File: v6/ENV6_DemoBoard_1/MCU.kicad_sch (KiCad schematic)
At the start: 44 parts, among them J1 Pico Debugger (SWD), J201 Conn_01x04, U101 RP2354B, U102 W25Q16JVUXIQ, U103 Pi-Radio, Y101 KX7_QRZ

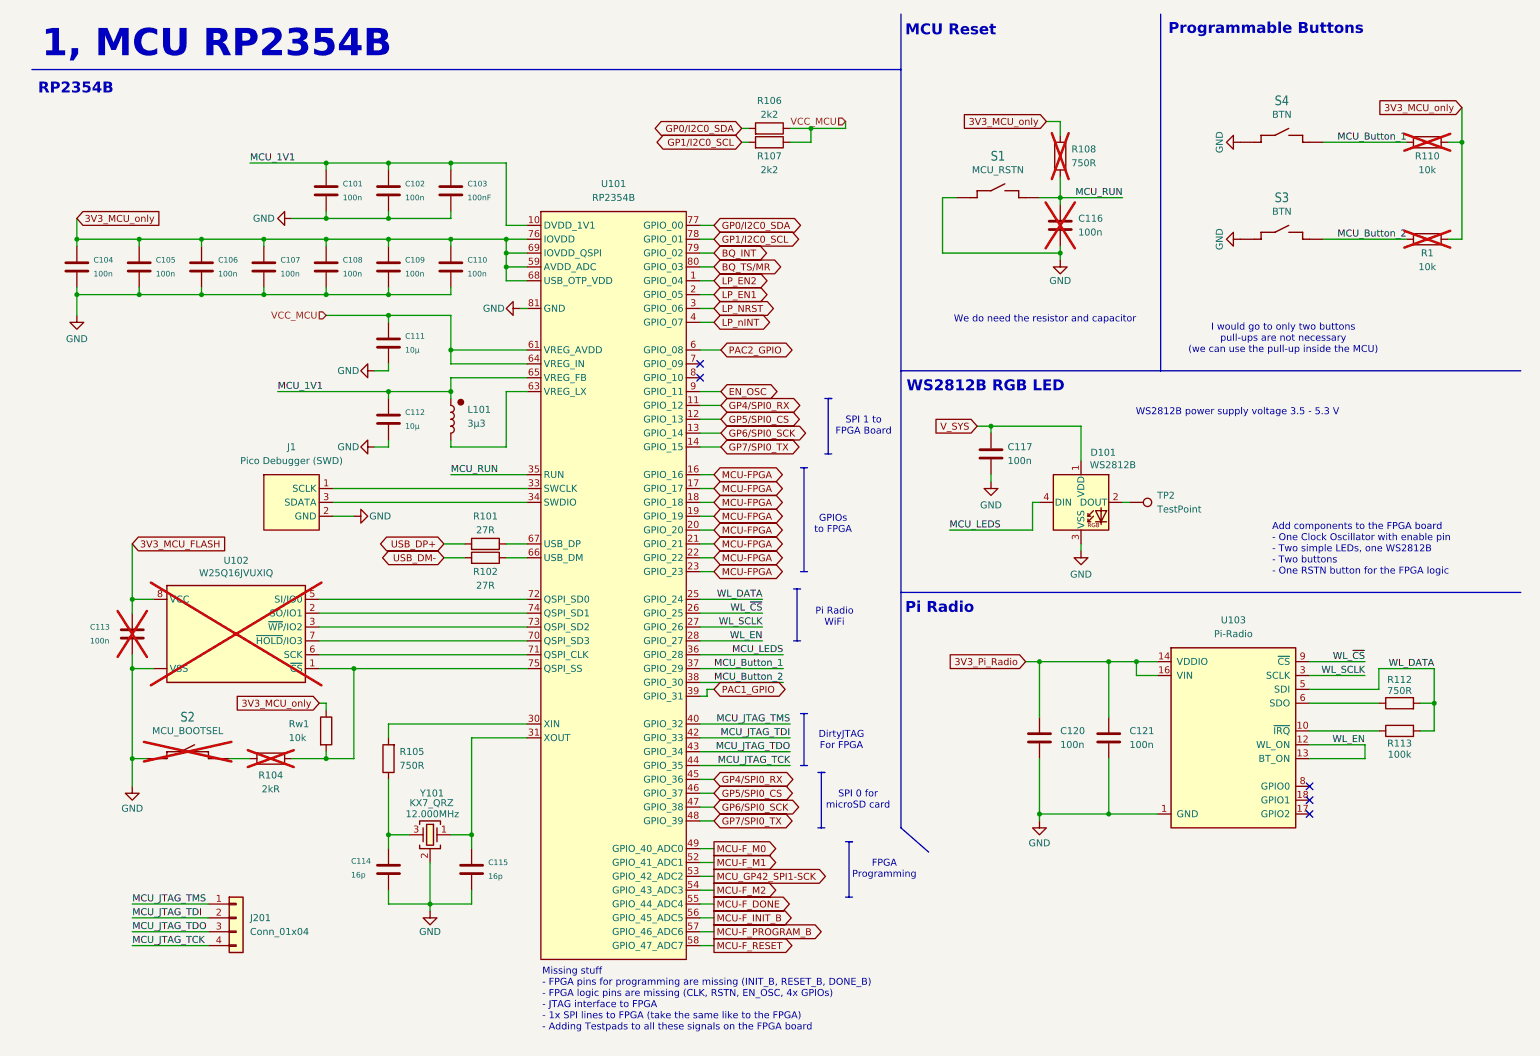
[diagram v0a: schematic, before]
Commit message: Changes after second rev of ENV6 test
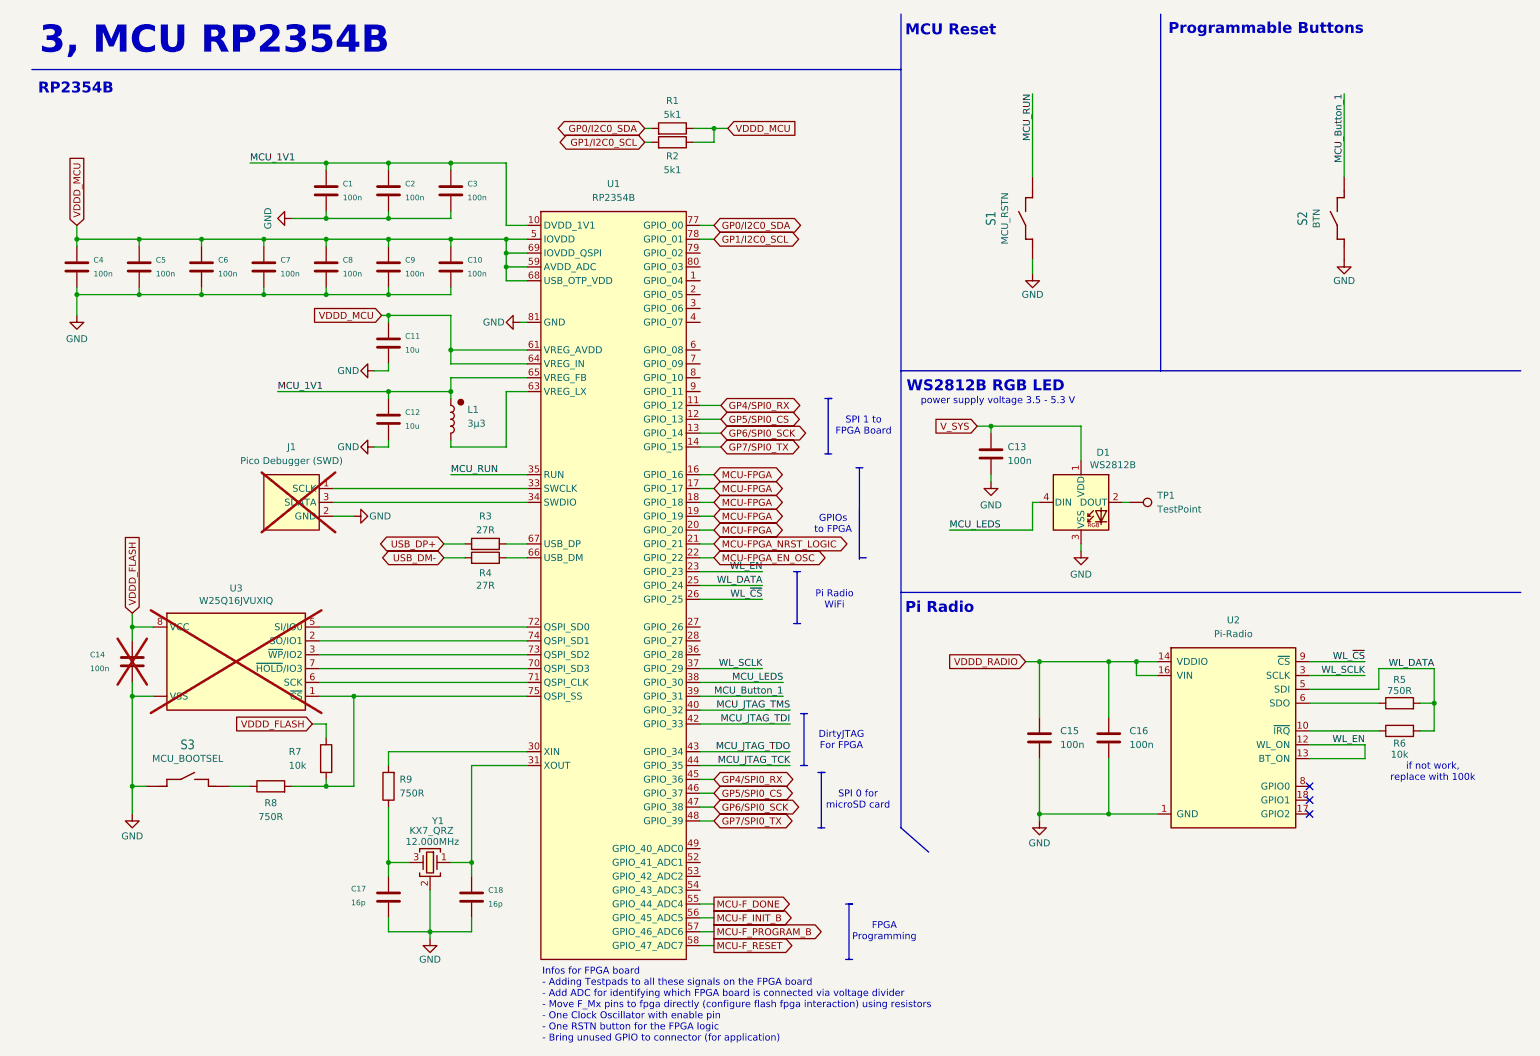
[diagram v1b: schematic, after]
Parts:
- removed C116: 100n, Capacitor_SMD:C_0402_1005Metric, symbol Device:C
- removed J201: Conn_01x04, Connector_PinHeader_2.54mm:PinHeader_1x04_P2.54mm_Vertical, symbol Connector_Generic:Conn_01x04
- removed R1, R110: 10k, Resistor_SMD:R_0402_1005Metric, symbol Device:R
- removed R108: 750R, Resistor_SMD:R_0402_1005Metric, symbol Device:R
- removed S3: BTN, connectors:TACTILE-SWITCH, symbol connectors:Tactile Button
- C11: renamed from C111; value 10µ -> 10u
- C12: renamed from C112; value 10µ -> 10u
- C3: renamed from C103; value 100nF -> 100n
- J1: now not fitted; now left out of the parts list
- R1: renamed from R106; value 2k2 -> 5k1
- R2: renamed from R107; value 2k2 -> 5k1
- R6: renamed from R113; value 100k -> 10k
- R8: renamed from R104; value 2kR -> 750R; now fitted; now in the parts list
- S3: renamed from S2; now fitted; now in the parts list
- renumbered C101 to C1, C110 to C10, C117 to C13, C113 to C14, C120 to C15, C121 to C16, C114 to C17, C115 to C18, C102 to C2, C104 to C4, C105 to C5, C106 to C6, C107 to C7, C108 to C8, C109 to C9, D101 to D1, L101 to L1, R101 to R3, R102 to R4, R112 to R5, Rw1 to R7, R105 to R9, S4 to S2, TP2 to TP1, U101 to U1, U103 to U2, U102 to U3, Y101 to Y1
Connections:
- net MCU_Button_2 is gone; now on net MCU_LEDS: U1.38 (GPIO_30)
- net PAC1_GPIO is gone; now on net MCU_Button_1: U1.39 (GPIO_31)
- net VCC_MCU is gone; now on net VDDD_MCU: C11.2, R1.1, R2.1, U1.61 (VREG_AVDD), U1.64 (VREG_IN)
- net MCU-FPGA: no longer U1.21 (GPIO_21), U1.22 (GPIO_22), U1.23 (GPIO_23)
- net MCU_Button_1: no longer U1.37 (GPIO_29)
- net MCU_LEDS: no longer U1.36 (GPIO_28)
- net WL_EN: now also U1.23 (GPIO_23); no longer U1.28 (GPIO_27)
- net WL_SCLK: now also U1.37 (GPIO_29); no longer U1.27 (GPIO_26)
- net 3V3_MCU_FLASH renamed VDDD_FLASH
- net VDDD_FLASH: now also R7.1
- net 3V3_Pi_Radio renamed VDDD_RADIO
- net BQ_INT: no longer names the net of U1.79 (GPIO_02)
- net BQ_TS/MR: no longer names the net of U1.80 (GPIO_03)
- net EN_OSC: no longer names the net of U1.9 (GPIO_11)
- net IOVDD renamed VDDD_MCU
- net VDDD_MCU: no longer R7.1
- net LP_EN1: no longer names the net of U1.2 (GPIO_05)
- net LP_EN2: no longer names the net of U1.1 (GPIO_04)
- net LP_NRST: no longer names the net of U1.3 (GPIO_06)
- net LP_nINT: no longer names the net of U1.4 (GPIO_07)
- net MCU-F_M0: no longer names the net of U1.49 (GPIO_40_ADC0)
- net MCU-F_M1: no longer names the net of U1.52 (GPIO_41_ADC1)
- net MCU-F_M2: no longer names the net of U1.54 (GPIO_43_ADC3)
- net MCU_GP42_SPI1-SCK: no longer names the net of U1.53 (GPIO_42_ADC2)
- net PAC2_GPIO: no longer names the net of U1.6 (GPIO_08)
- new net MCU-FPGA_EN_OSC: U1.22 (GPIO_22)
- new net MCU-FPGA_NRST_LOGIC: U1.21 (GPIO_21)
- no-connect marks 5 -> 3
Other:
- note added: "3, MCU RP2354B"
- note added: "Infos for FPGA board - Adding Testpads to all these signals on the FPGA board - Add ADC for identifying which FPGA board is connected via voltage divider - Move F_Mx pins to fpga directly (configure flash fpga interaction) using resistors - One Clock Oscillator with enable pin - One RSTN button for the FPGA logic - Bring unused GPIO to connector (for application)"
- note added: "if not work, replace with 100k"
- note added: "power supply voltage 3.5 - 5.3 V"
- note removed: "1, MCU RP2354B"
- note removed: "Add components to the FPGA board - One Clock Oscillator with enable pin - Two simple LEDs, one WS2812B - Two buttons - One RSTN button for the FPGA logic"
- note removed: "I would go to only two buttons pull-ups are not necessary (we can use the pull-up inside the MCU)"
- note removed: "Missing stuff - FPGA pins for programming are missing (INIT_B, RESET_B, DONE_B) - FPGA logic pins are missing (CLK, RSTN, EN_OSC, 4x GPIOs) - JTAG interface to FPGA - 1x SPI lines to FPGA (take the same like to the FPGA) - Adding Testpads to all these signals on the FPGA board"
- note removed: "WS2812B power supply voltage 3.5 - 5.3 V"
- note removed: "We do need the resistor and capacitor"
- moved on the sheet: C14, C17, C18, R1, R2, R7, R9, S1, S2, U3, Y1
